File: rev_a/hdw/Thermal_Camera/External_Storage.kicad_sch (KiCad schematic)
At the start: 44 parts

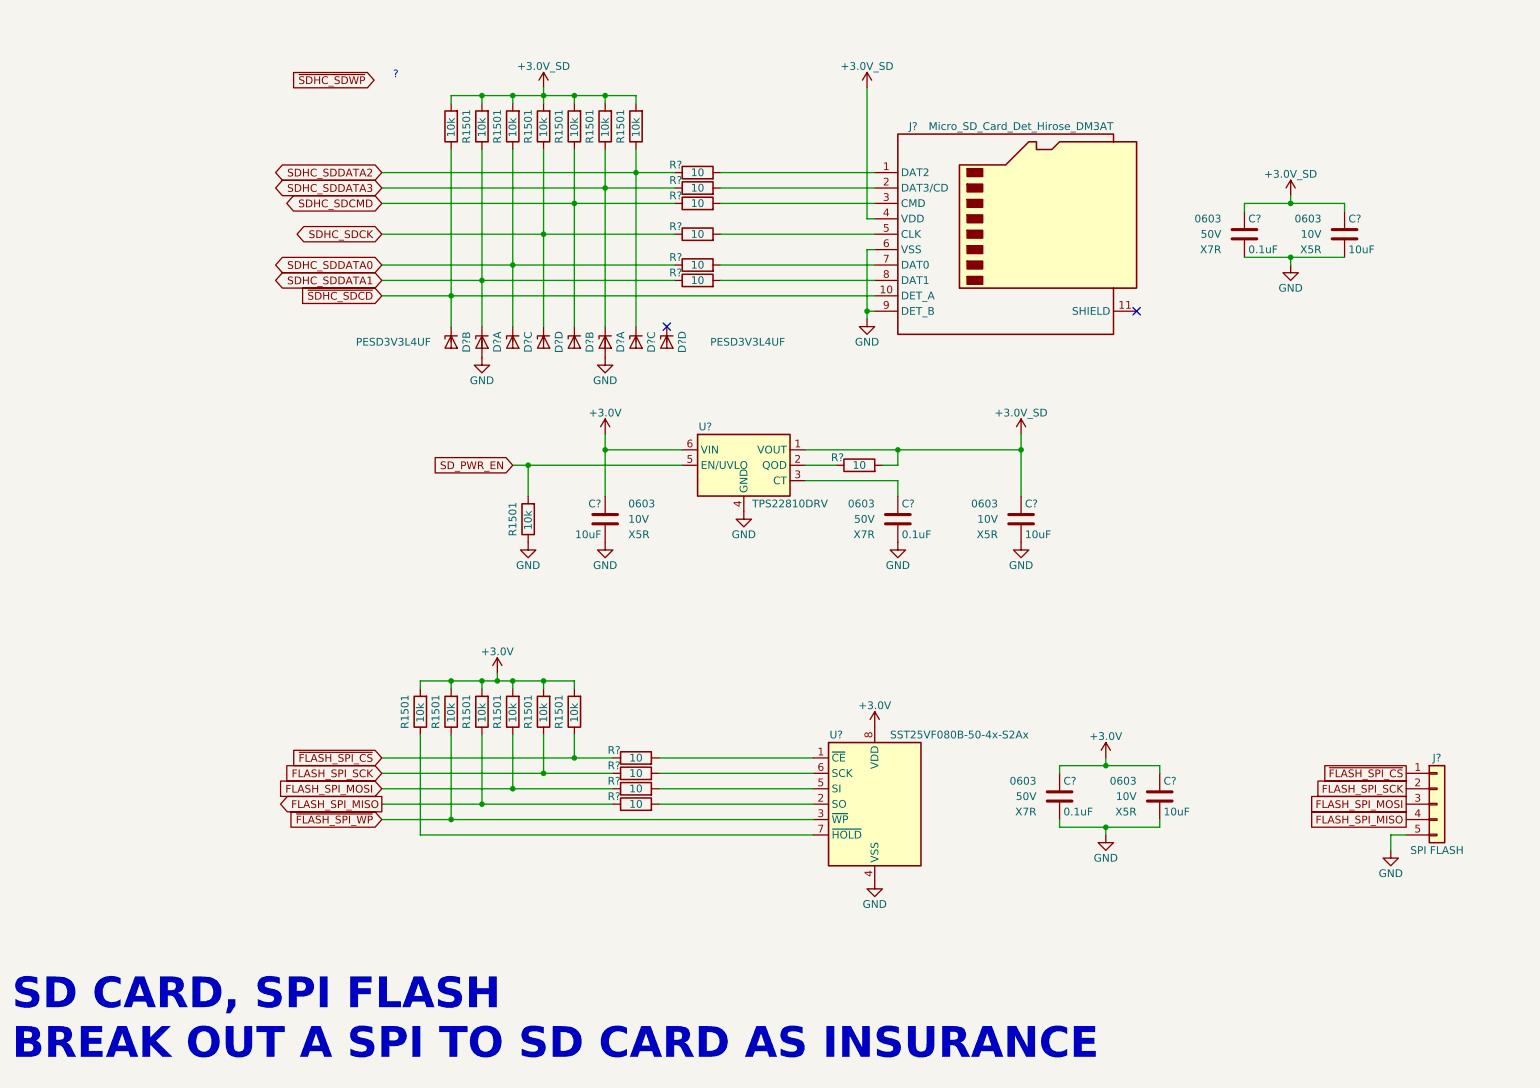
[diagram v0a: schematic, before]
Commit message: lots of random schematic progress
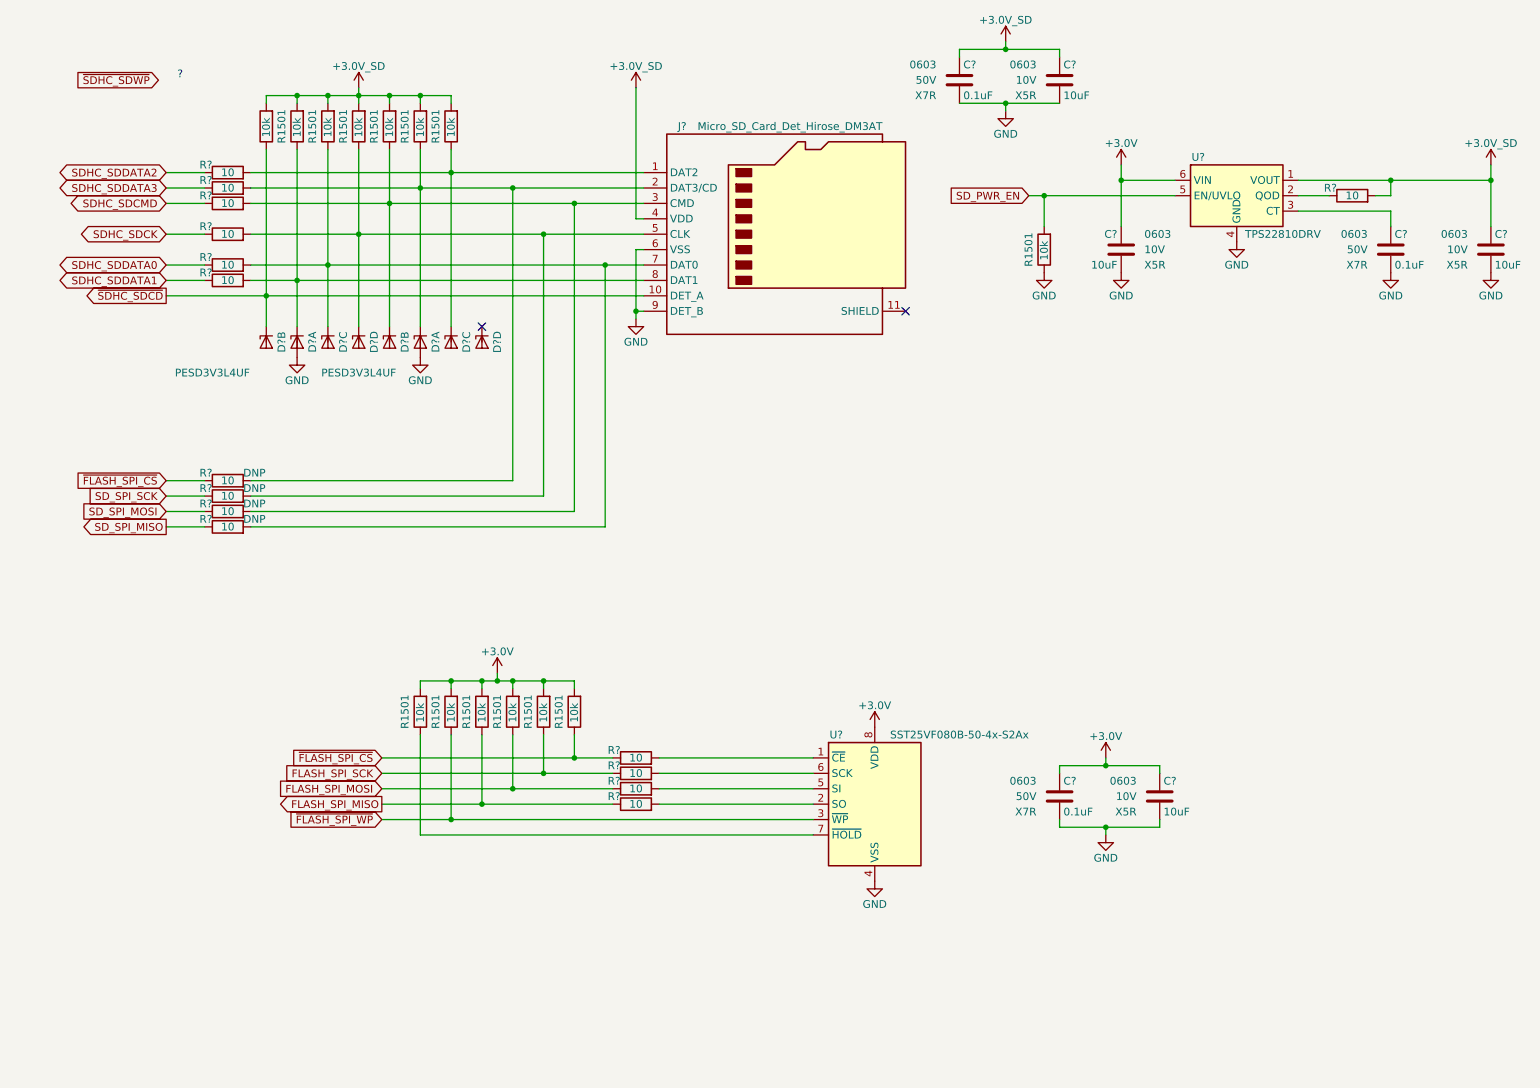
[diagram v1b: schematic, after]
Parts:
- removed J?: SPI FLASH, symbol Connector_Generic:Conn_01x05
- added R? (x4): 10, Resistors_SMD:R_0603, symbol Custom_Library:R_Custom
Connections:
- net SDHC_SDCK: no longer D?.6 (K4), R1501.2
- net SDHC_SDCMD: no longer D?.3 (K2), R1501.2
- net SDHC_SDDATA0: no longer D?.4 (K3), R1501.2
- net SDHC_SDDATA1: no longer D?.1 (K1), R1501.2
- net SDHC_SDDATA2: no longer D?.4 (K3), R1501.2
- net SDHC_SDDATA3: no longer D?.1 (K1), R1501.2
- net ~{FLASH_SPI_CS}: now also R?.2
- net at J?.1 (DAT2), R?.1: now also D?.4 (K3), R1501.2
- net at J?.2 (DAT3/CD), R?.1: now also D?.1 (K1), R1501.2, R?.1
- net at J?.3 (CMD), R?.1: now also D?.3 (K2), R1501.2, R?.1
- net at J?.5 (CLK), R?.1: now also D?.6 (K4), R1501.2, R?.1
- net at J?.7 (DAT0), R?.1: now also D?.4 (K3), R1501.2, R?.1
- net at J?.8 (DAT1), R?.1: now also D?.1 (K1), R1501.2
- new net SD_SPI_MISO: R?.2
- new net SD_SPI_MOSI: R?.2
- new net SD_SPI_SCK: R?.2
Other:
- note removed: "SD CARD, SPI FLASH BREAK OUT A SPI TO SD CARD AS INSURANCE"
- moved on the sheet: C?, D?A, D?B, D?C, D?D, J?, R1501, R?, U?
